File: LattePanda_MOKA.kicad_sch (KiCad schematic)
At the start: 6 parts

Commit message: hierarchical schema rework
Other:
- sheet CSI ports: added CSI_C{CSI}, CSI_D{CSI}; removed CSI_C_CK+, CSI_C_CK-, CSI_C_D0+, CSI_C_D0-, CSI_C_D1+, CSI_C_D1-, CSI_C_D2+, CSI_C_D2-, CSI_C_D3+, CSI_C_D3-, CSI_D_CK+, CSI_D_CK-, DPHY0_C{DPHY}
- sheet GPIO ports: added none; removed I2C4_SCL, I2C4_SDA, I2C5_SCL, I2C5_SDA, SOC_UART0_RX, SOC_UART0_TX, SOC_UART1_RX, SOC_UART1_TX, SOC_UART2_RX, SOC_UART2_TX
- sheet Gigabit Ethernet ports: added GBE{GBE}; removed GbE_PCIe_CLK+, GbE_PCIe_CLK-, GbE_PCIe_RX+, GbE_PCIe_RX-, GbE_PCIe_TX+, GbE_PCIe_TX-
- sheet HDMI ports: added HDMI_1{HDMI}; removed DDI_B_TX0+, DDI_B_TX0-, DDI_B_TX1+, DDI_B_TX1-, DDI_B_TX2+, DDI_B_TX2-, DDI_B_TX3+, DDI_B_TX3-
- sheet LattePanda Module ports: added CSI_C{CSI}, CSI_D{CSI}, GBE{GBE}, HDMI_1{HDMI}, PCIE_2{PCIE}, PCIE_3{PCIE}, USB2_3{USB}, USB2_5{USB}, USB3_2{USB}; removed CSI_C_CK+, CSI_C_CK-, CSI_C_D0+, CSI_C_D0-, CSI_C_D1+, CSI_C_D1-, CSI_C_D2+, CSI_C_D2-, CSI_C_D3+, CSI_C_D3-, CSI_D_CK+, CSI_D_CK-, DDI_B_TX0+, DDI_B_TX0-, DDI_B_TX1+, DDI_B_TX1-, DDI_B_TX2+, DDI_B_TX2-, DDI_B_TX3+, DDI_B_TX3-, HSIO_0_RX+, HSIO_0_RX-, HSIO_0_TX+, HSIO_0_TX-, HSIO_1_RX+, HSIO_1_RX-, HSIO_1_TX+, HSIO_1_TX-, HSIO_2_RX+, HSIO_2_RX-, HSIO_2_TX+, HSIO_2_TX-, HSIO_3_RX+, HSIO_3_RX-, HSIO_3_TX+, HSIO_3_TX-, HSIO_6_RX+, HSIO_6_RX-, HSIO_6_TX+, HSIO_6_TX-, I2C4_SCL, I2C4_SDA, REFCLK0+, REFCLK0-, REFCLK3+, REFCLK3-, REFCLK4+, REFCLK4-, SOC_UART0_RX, SOC_UART0_TX, SOC_UART1_RX, SOC_UART1_TX, SOC_UART2_RX, SOC_UART2_TX, USB_2_P1+, USB_2_P1-, USB_2_P2+, USB_2_P2-, USB_2_P3+, USB_2_P3-, USB_2_P5+, USB_2_P5-, USB_2_P7+, USB_2_P7-
- sheet M.2 E&M Key ports: added PCIE_E{PCIE}, PCIE_M{PCIE}; removed PCIE_RX_0+, PCIE_RX_0-, PCIE_RX_1+, PCIE_RX_1-, PCIE_TX_0+, PCIE_TX_0-, PCIE_TX_1+, PCIE_TX_1-, REFCLKE+, REFCLKE-, REFCLKM+, REFCLKM-, USB_2_P7+, USB_2_P7-
- sheet USB2.0&USB3.0 ports: added USB2_3{USB}, USB2_5{USB}, USB3{USB}; removed USB3_SSRX_N, USB3_SSRX_P, USB3_SSTX_N, USB3_SSTX_P, USB4_SSRX_N, USB4_SSRX_P, USB4_SSTX_N, USB4_SSTX_P, USB_2_P1+, USB_2_P1-, USB_2_P2+, USB_2_P2-, USB_2_P3+, USB_2_P3-, USB_2_P5+, USB_2_P5-
- note added: "[MOKA - MINI LATTEPANDA MU CARRIER BOARD]"
- moved on the sheet: FID1, FID2, H1, H2, H3, H4

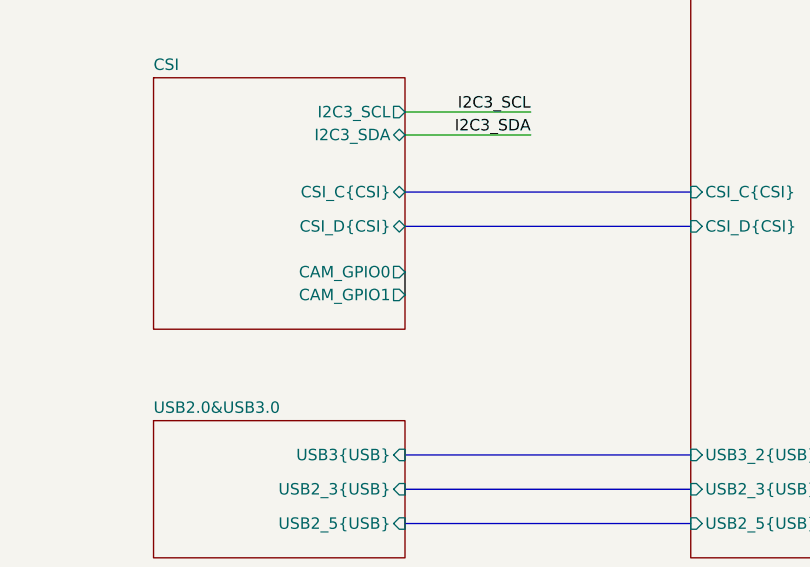
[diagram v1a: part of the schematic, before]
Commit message: save
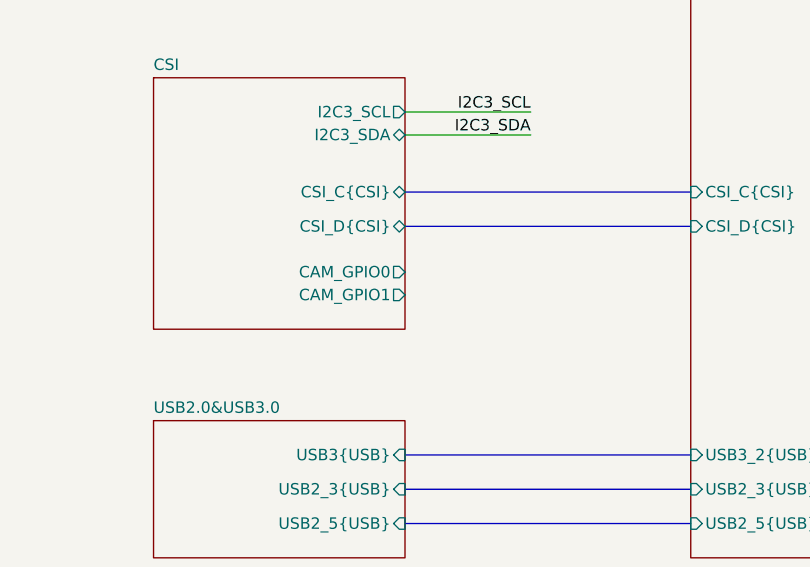
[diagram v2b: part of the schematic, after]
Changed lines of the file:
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@@
-	(wire
-		(pts
-			(xy 86.36 124.46) (xy 86.36 127)
-		)
-		(stroke
-			(width 0)
-			(type default)
-		)
-	)
 	(wire
 		(pts
